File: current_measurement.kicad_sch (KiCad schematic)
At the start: 15 parts, among them J1 Conn_01x02_Male, J2 Conn_01x02_Female, J3 Conn_01x02_Male, J4 USB_B_Micro, U1 MAX680CSA+T, U2 INA105

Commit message: v1.1: SOC package for MAX680
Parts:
- U1: footprint Package_DIP:DIP-8_W7.62mm -> Package_SO:SOIC-8_3.9x4.9mm_P1.27mm
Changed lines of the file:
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@@
     (title "Current Measurement")
     (date "2022-12-01")
-    (rev "1.0")
+    (rev "1.1")
     (company "Christian Eisendle")
   )
@@
     (property "Reference" "U1" (id 0) (at 87.63 59.69 0))
     (property "Value" "MAX680CSA+T" (id 1) (at 87.63 62.23 0))
-    (property "Footprint" "Package_DIP:DIP-8_W7.62mm" (id 2) (at 73.66 57.15 0)
+    (property "Footprint" "Package_SO:SOIC-8_3.9x4.9mm_P1.27mm" (id 2) (at 73.66 57.15 0)
       (effects (font (size 1.27 1.27)) (justify left) hide)
     )
@@
     )
     (path "/1de28cda-4d36-41c8-83c0-b9aade470c4f"
-      (reference "U1") (unit 1) (value "MAX680CSA+T") (footprint "Package_DIP:DIP-8_W7.62mm")
+      (reference "U1") (unit 1) (value "MAX680CSA+T") (footprint "Package_SO:SOIC-8_3.9x4.9mm_P1.27mm")
     )
     (path "/084b112d-dcfd-4801-aa54-60bf427059e5"

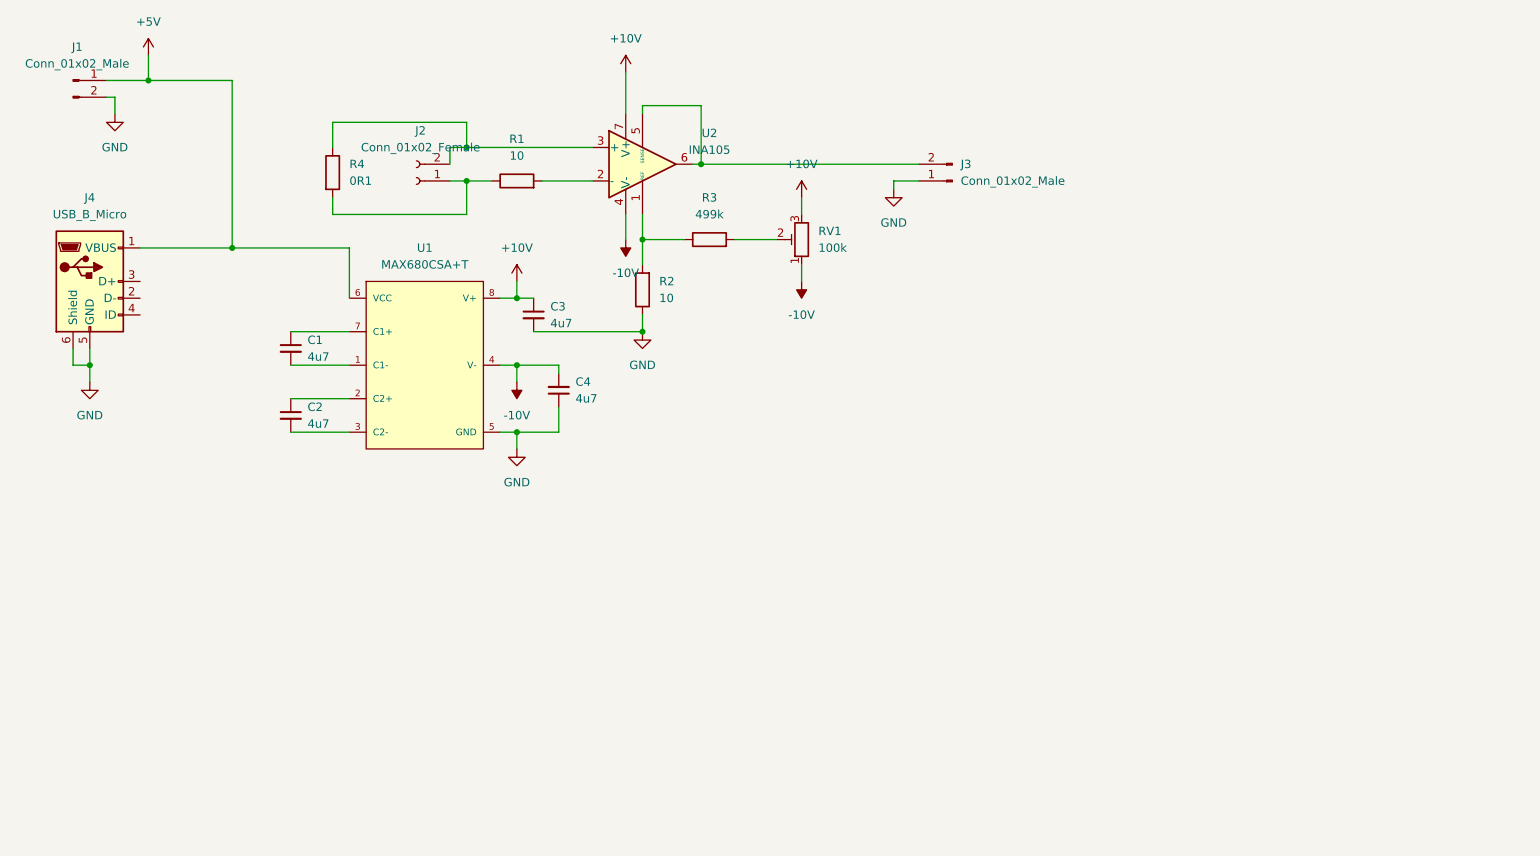
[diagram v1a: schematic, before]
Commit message: Current Shunt 2.0
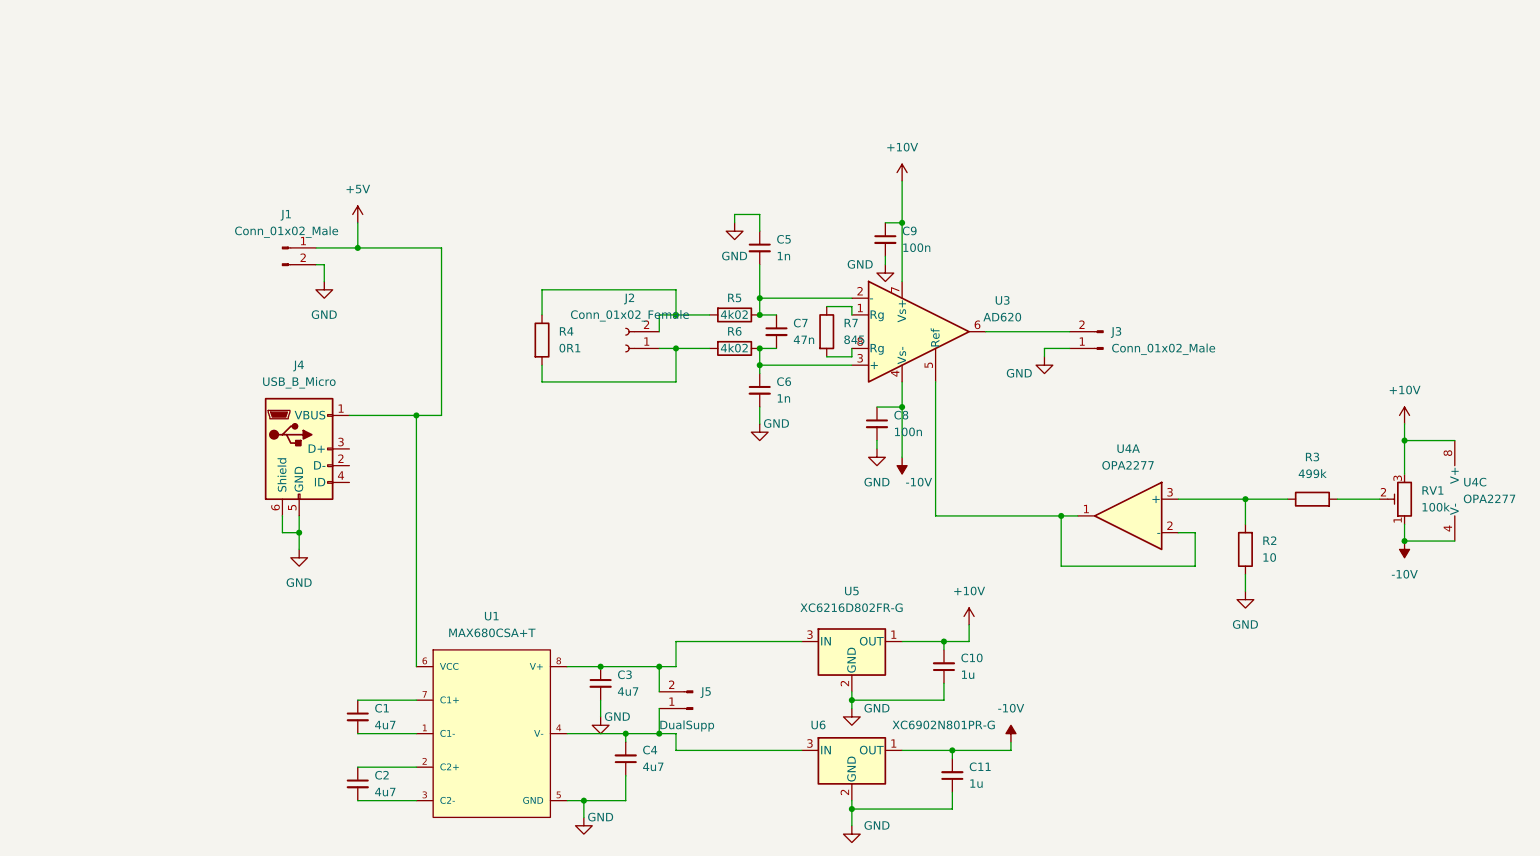
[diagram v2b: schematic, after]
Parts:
- removed R1: 10, Resistor_SMD:R_0402_1005Metric_Pad0.72x0.64mm_HandSolder, symbol Device:R
- removed U2: INA105, Package_SO:SOIC-8_3.9x4.9mm_P1.27mm, symbol Amplifier_Difference:AD8276
- added C10, C11: 1u, Capacitor_SMD:C_0402_1005Metric_Pad0.74x0.62mm_HandSolder, symbol Device:C_Small
- added C5, C6: 1n, Capacitor_SMD:C_0402_1005Metric_Pad0.74x0.62mm_HandSolder, symbol Device:C_Small
- added C7: 47n, Capacitor_SMD:C_0402_1005Metric_Pad0.74x0.62mm_HandSolder, symbol Device:C_Small
- added C8, C9: 100n, Capacitor_SMD:C_0603_1608Metric, symbol Device:C_Small
- added J5: DualSupp, Connector_PinHeader_2.54mm:PinHeader_1x02_P2.54mm_Vertical, symbol Connector:Conn_01x02_Male
- added R5, R6: 4k02, Resistor_SMD:R_0402_1005Metric_Pad0.72x0.64mm_HandSolder, symbol Device:R
- added R7: 845, Resistor_SMD:R_0402_1005Metric_Pad0.72x0.64mm_HandSolder, symbol Device:R
- added U3: AD620, Package_SO:SOIC-8_3.9x4.9mm_P1.27mm, symbol Amplifier_Instrumentation:AD620
- added U4: OPA2277, Package_SO:SOIC-8_3.9x4.9mm_P1.27mm, symbol Amplifier_Operational:OPA2277
- added U5: XC6216D802FR-G, Package_TO_SOT_SMD:SOT-223-3_TabPin2, symbol Regulator_Linear:MCP1804x-C002xDB
- added U6: XC6902N801PR-G, Package_TO_SOT_SMD:SOT-223-3_TabPin2, symbol Regulator_Linear:MCP1804x-C002xDB
- C1, C2, C3, C4: footprint Capacitor_SMD:CP_Elec_4x5.8 -> Capacitor_SMD:C_1210_3225Metric
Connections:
- net +10V: now also C10.2, C9.1, U3.7 (Vs+), U4.8 (V+), U5.1 (OUT); no longer C3.1, U1.8 (V+)
- net -10V: now also C11.2, C8.1, U3.4 (Vs-), U4.4 (V-), U6.1 (OUT); no longer C4.2, U1.4 (V-)
- net GND: now also C10.1, C11.1, C5.1, C6.2, C8.2, C9.2, U5.2 (GND), U6.2 (GND)
- net at R2.2, R3.1: now also U4.3 (+)
- net at J2.2 (Pin_2), R4.1: now also R5.2
- net at J3.2 (Pin_2): now also U3.6
- net at J2.1 (Pin_1), R4.2: now also R6.2
- new net: C3.1, J5.2 (Pin_2), U1.8 (V+), U5.3 (IN)
- new net: C5.2, C7.1, R5.1, U3.2 (-)
- new net: C4.2, J5.1 (Pin_1), U1.4 (V-), U6.3 (IN)
- new net: U3.5 (Ref), U4.1, U4.2 (-)
- new net: R7.1, U3.1 (Rg)
- new net: R7.2, U3.8 (Rg)
- new net: C6.1, C7.2, R6.1, U3.3 (+)
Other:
- moved on the sheet: C1, C2, C3, C4, J1, J2, J3, J4, R2, R3, R4, RV1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
